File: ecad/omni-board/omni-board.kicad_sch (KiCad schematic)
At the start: 5 parts, among them J1 Motor_BTS7960_01, J2 Motor_BTS7960_02, J3 Motor_BTS7960_03, J4 Motor_BTS7960_04, U2 ESP32-S3-DevKitC

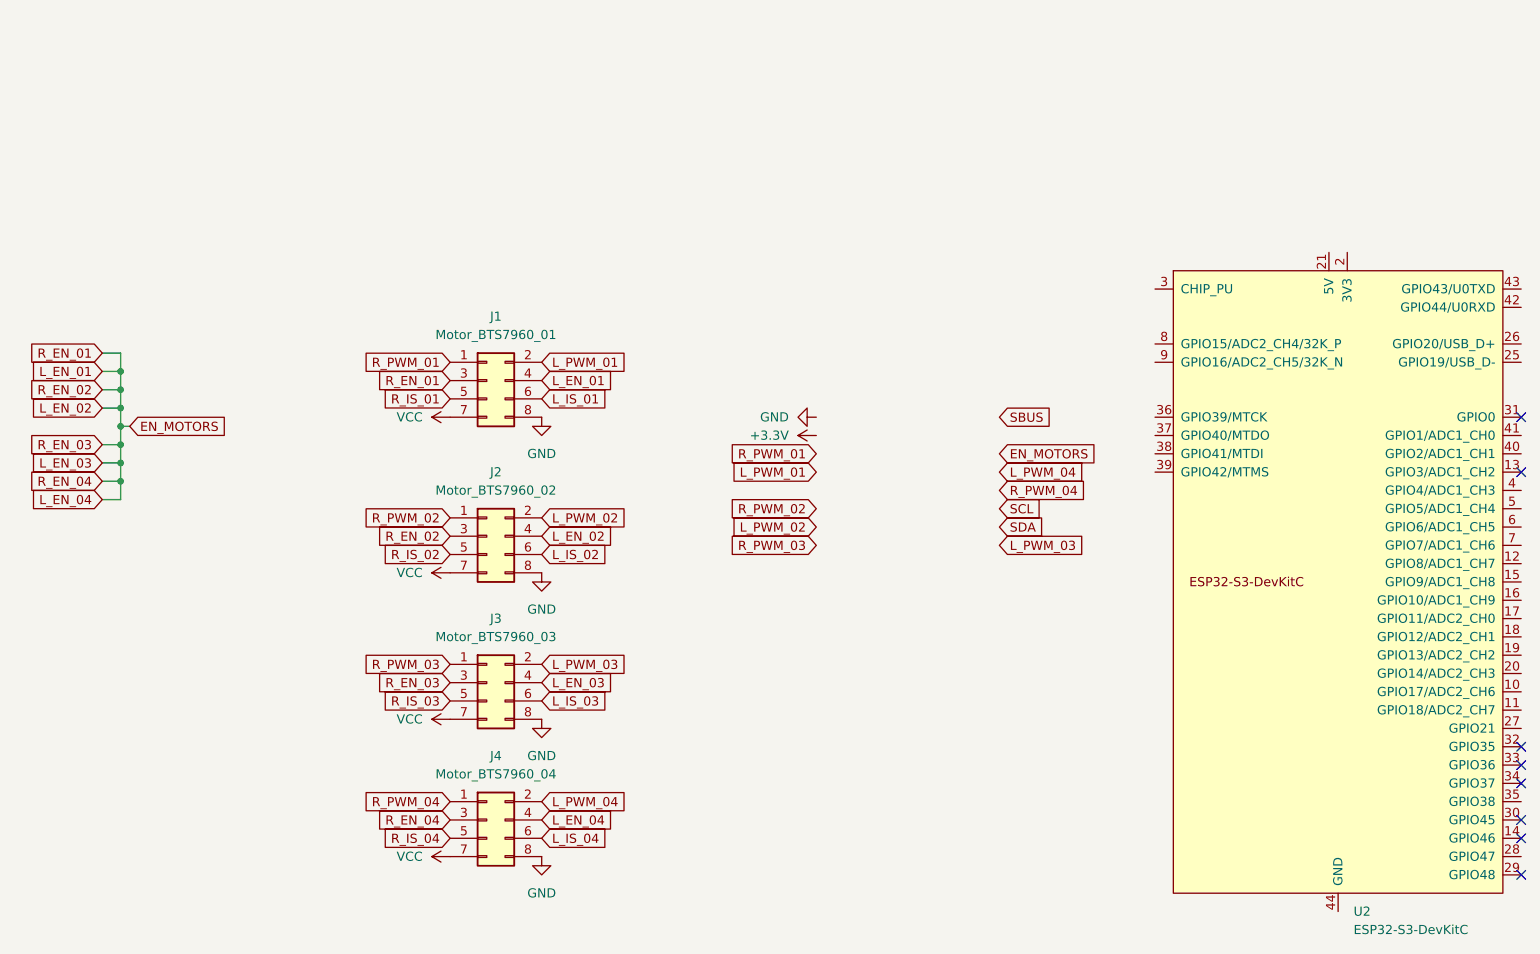
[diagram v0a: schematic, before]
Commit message: update for production
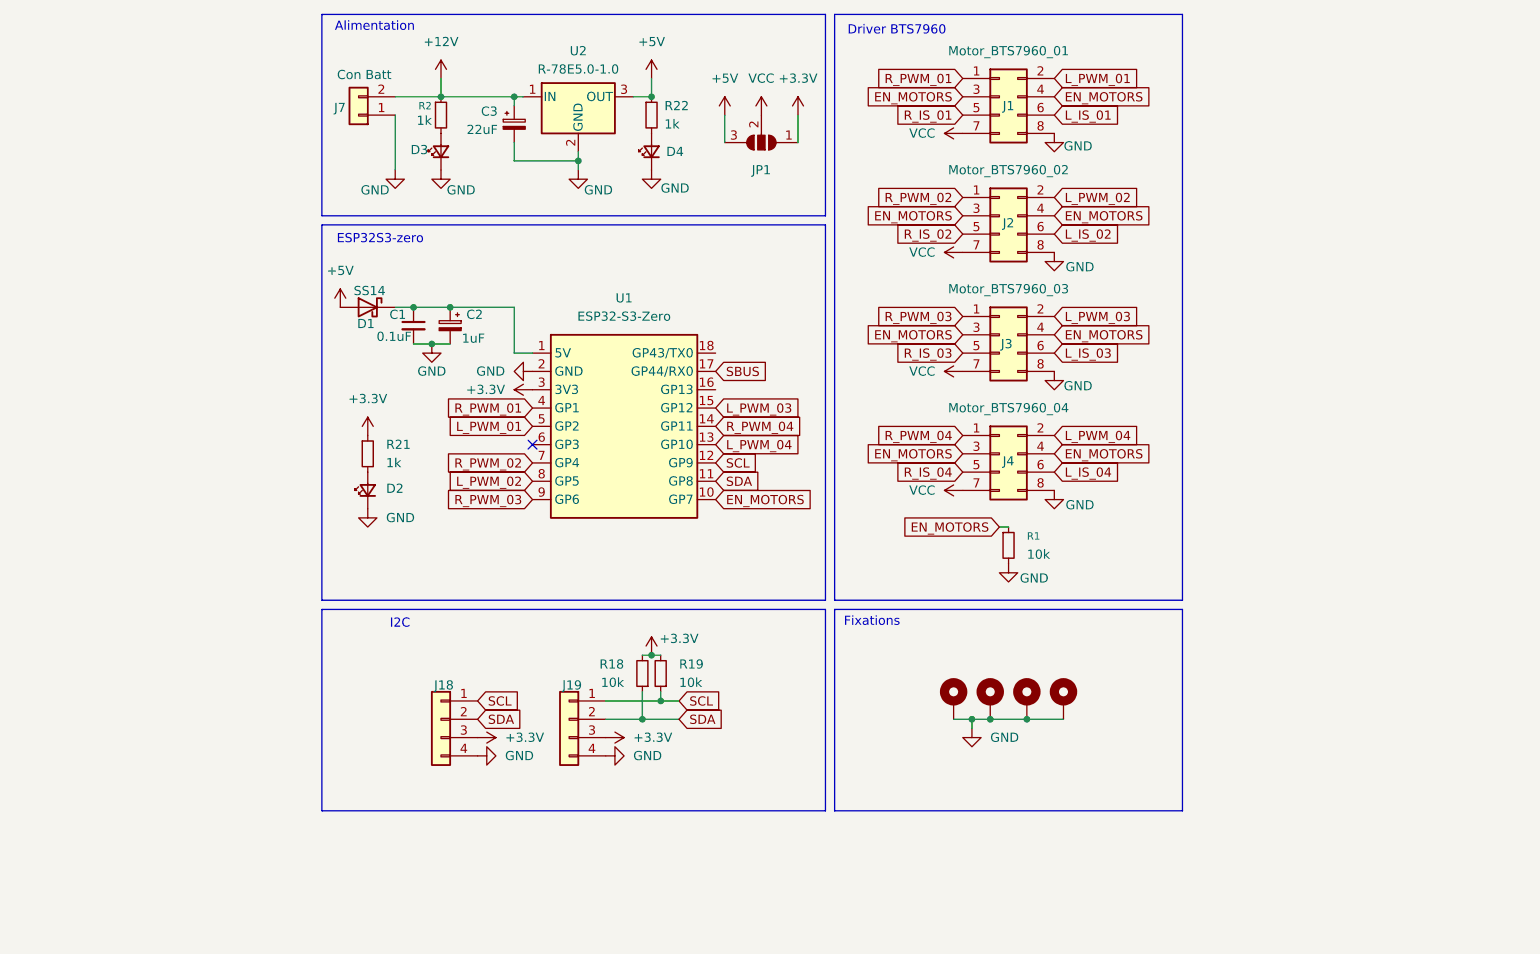
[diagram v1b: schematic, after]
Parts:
- removed U2: ESP32-S3-DevKitC, PCM_Espressif:ESP32-S3-DevKitC, symbol PCM_Espressif:ESP32-S3-DevKitC
- added C1: 0.1uF, Capacitor_SMD:C_1206_3216Metric_Pad1.33x1.80mm_HandSolder, symbol Device:C_Small
- added C2: 1uF, Capacitor_SMD:CP_Elec_5x5.4, symbol Device:C_Polarized_Small
- added C3: 22uF, Capacitor_SMD:CP_Elec_5x5.4, symbol Device:C_Polarized_Small
- added D1: SS14, Diode_SMD:D_SMA_Handsoldering, symbol Diode:SS14
- added D2, D3, D4: LED_Small, LED_SMD:LED_1206_3216Metric_Pad1.42x1.75mm_HandSolder, symbol Device:LED_Small
- added H1, H2, H3, H4: MountingHole_Pad, MountingHole:MountingHole_3.2mm_M3_Pad_Via, symbol Mechanical:MountingHole_Pad
- added J18, J19: Conn_01x04, Connector_Molex:Molex_KK-254_AE-6410-04A_1x04_P2.54mm_Vertical, symbol Connector_Generic:Conn_01x04
- added J7: Con Batt, Connector_AMASS:AMASS_XT60-M_1x02_P7.20mm_Vertical, symbol Connector_Generic:Conn_01x02
- added JP1: SolderJumper_3_Open, Jumper:SolderJumper-3_P2.0mm_Open_TrianglePad1.0x1.5mm, symbol Jumper:SolderJumper_3_Open
- added R1, R18, R19: 10k, Resistor_SMD:R_1206_3216Metric_Pad1.30x1.75mm_HandSolder, symbol Device:R_Small
- added R2, R21, R22: 1k, Resistor_SMD:R_1206_3216Metric_Pad1.30x1.75mm_HandSolder, symbol Device:R_Small
- added U1: ESP32-S3-Zero, omni-footprints:ESP32-S3-Zero_THT, symbol omni-symbols:ESP32-S3-Zero
- added U2: R-78E5.0-1.0, Converter_DCDC:Converter_DCDC_RECOM_R-78E-0.5_THT, symbol Converter_DCDC:R-78E5.0-1.0
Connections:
- net +3.3V: now also J18.3 (Pin_3), J19.3 (Pin_3), JP1.1 (A), R18.2, R19.2, R21.1, U1.3 (3V3)
- net EN_MOTORS: now also R1.1, U1.10 (GP7)
- net GND: now also C1.2, C2.2, C3.2, D2.1 (K), D3.1 (K), D4.1 (K), H1.1, H2.1, H3.1, H4.1, J18.4 (Pin_4), J19.4 (Pin_4), J7.1 (Pin_1), R1.2, U1.2 (GND), U2.2 (GND)
- net L_PWM_01: now also U1.5 (GP2)
- net L_PWM_02: now also U1.8 (GP5)
- net L_PWM_03: now also U1.15 (GP12)
- net L_PWM_04: now also U1.13 (GP10)
- net R_PWM_01: now also U1.4 (GP1)
- net R_PWM_02: now also U1.7 (GP4)
- net R_PWM_03: now also U1.9 (GP6)
- net R_PWM_04: now also U1.14 (GP11)
- net SBUS: now also U1.17 (GP44/RX0)
- net SCL: now also J18.1 (Pin_1), J19.1 (Pin_1), R19.1, U1.12 (GP9)
- net SDA: now also J18.2 (Pin_2), J19.2 (Pin_2), R18.1, U1.11 (GP8)
- net VCC: now also JP1.2 (C)
- new net: D2.2 (A), R21.2
- new net: C1.1, C2.1, D1.1 (K), U1.1 (5V)
- new net: D4.2 (A), R22.2
- new net: D3.2 (A), R2.2
- new net +12V: C3.1, J7.2 (Pin_2), R2.1, U2.1 (IN)
- new net +5V: D1.2 (A), JP1.3 (B), R22.1, U2.3 (OUT)
- no-connect marks 8 -> 1
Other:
- note added: "Alimentation"
- note added: "Driver BTS7960"
- note added: "ESP32S3-zero"
- note added: "Fixations"
- note added: "I2C"
- moved on the sheet: J1, J2, J3, J4
